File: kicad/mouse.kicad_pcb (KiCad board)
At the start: 2 copper layers, 100 x 100 mm, 49 parts, among them IC1 L7805, P1 SOURCE_12v, P10 LED_CONN, P11 SW_CONN, P12 LED_K_CONN, P15 UI_SOURCE, P16 LED_K_CONN, P17 LED_CONN, P18 SW_CONN, P2 SOURCE_12v, P3 battery 12v, P4 SOURCE_5v, P5 SOURCE_5v, P6 SOURCE_5v, P7 SOURCE_5v, P8 IR_CONN, P9 MOTOR_CONTROL, Q5 BSS138, Q6 BSS138, Q7 BSS138, SW1 SPST, SW2 SW_PUSH, SW3 SW_PUSH, SW4 SW_PUSH, SW5 SPST, U1 MCP3008

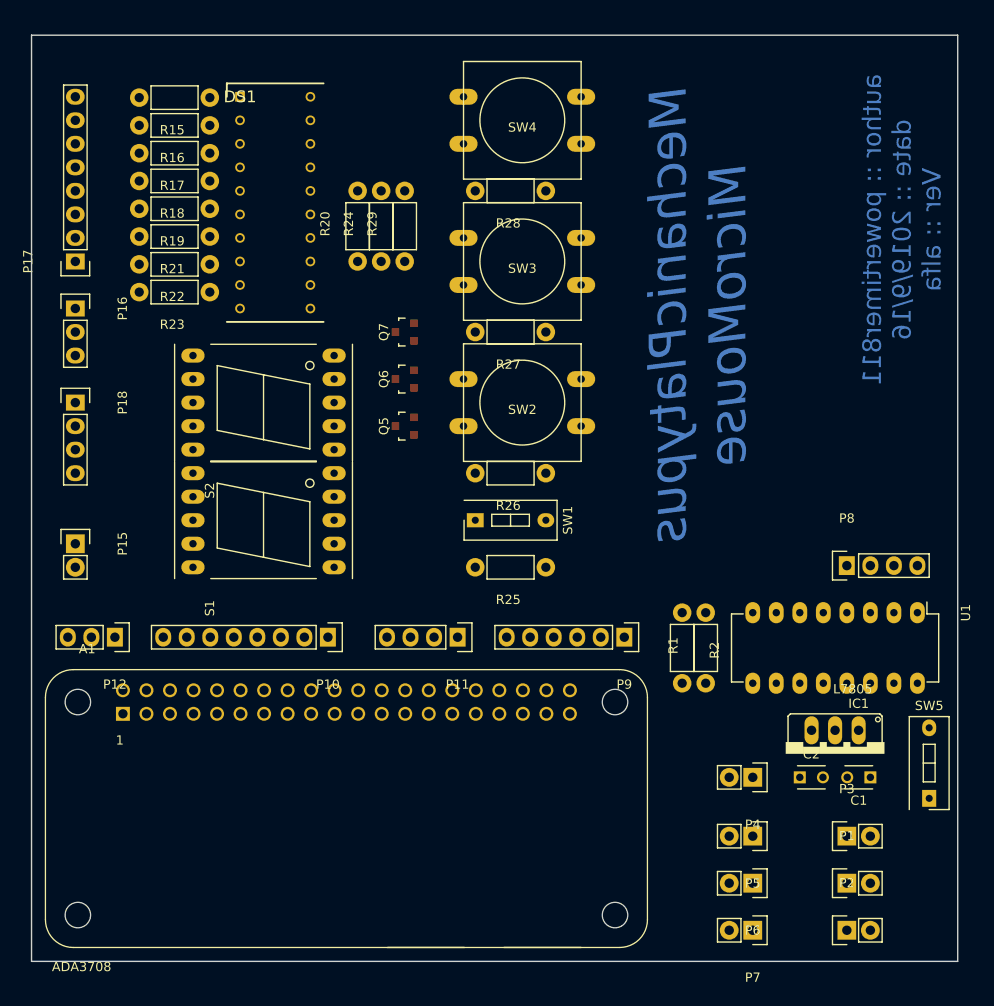
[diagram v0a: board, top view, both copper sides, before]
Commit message: complate kicad
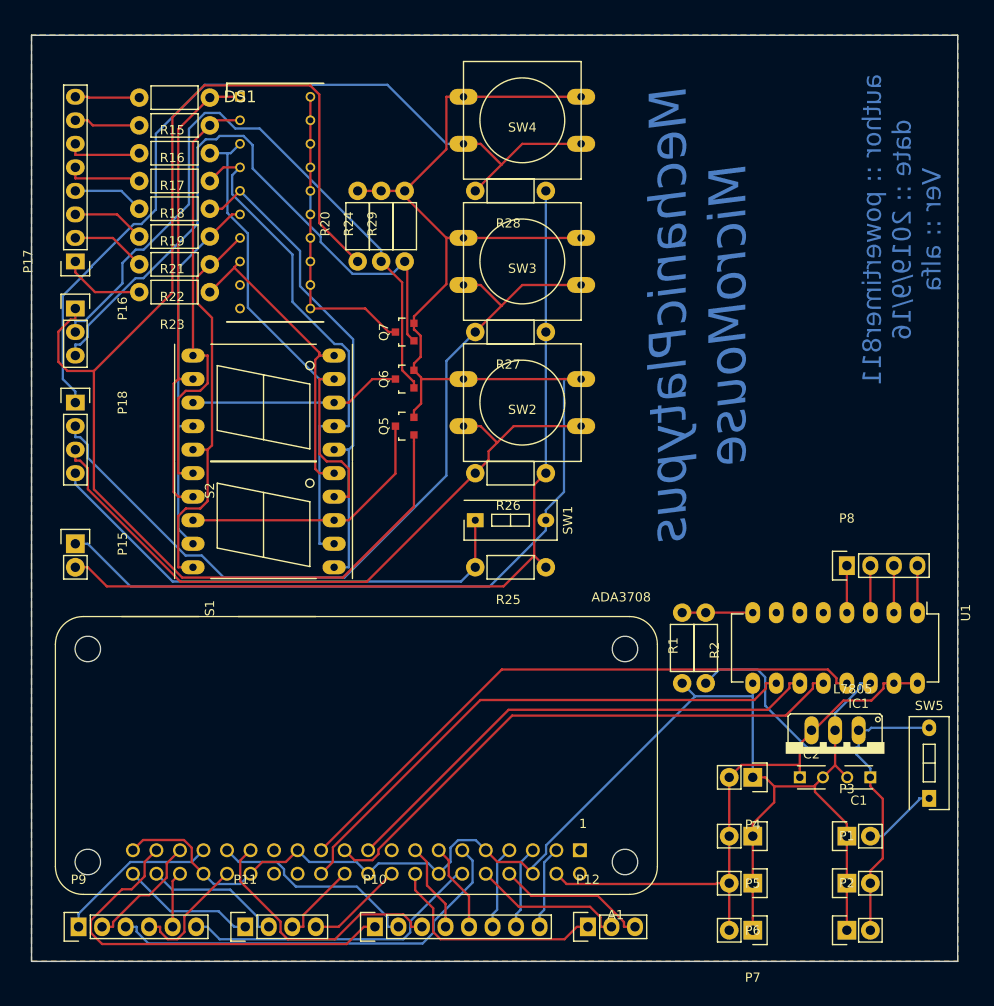
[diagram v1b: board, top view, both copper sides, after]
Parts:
- moved P9 66.7 mm to (30.1, 166.3), turned to 0 degrees
- moved P12 59.9 mm to (85.1, 166.3), turned to 0 degrees
- moved P11 38.8 mm to (48.1, 166.3), turned to 0 degrees
- moved P10 31.7 mm to (62.1, 166.3), turned to 0 degrees
- moved A1 17.3 mm to (60.1, 159.3), turned to 180 degrees
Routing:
- net Net-(P15-Pad1): track 0.00 -> 166.7 mm
- net GND: track 0.00 -> 155.4 mm
- net Net-(P16-Pad1): track 0.00 -> 141.6 mm
- net Net-(P15-Pad2): track 0.00 -> 93.4 mm
- net Net-(P18-Pad1): track 0.00 -> 90.8 mm
- net Net-(P18-Pad2): track 0.00 -> 88.3 mm
- net Net-(P18-Pad3): track 0.00 -> 74.4 mm
- net Net-(P16-Pad2): track 0.00 -> 72.1 mm
- net Net-(P16-Pad3): track 0.00 -> 69.1 mm
- net Net-(A1-Pad23): track 0.00 -> 65.8 mm
- net +5V: track 0.00 -> 63.4 mm
- net Net-(A1-Pad21): track 0.00 -> 60.7 mm
- net Net-(A1-Pad24): track 0.00 -> 58.9 mm
- net Net-(DS1-Pad4): track 0.00 -> 55.3 mm
- net Net-(P18-Pad4): track 0.00 -> 54.4 mm
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- added copper zone on B.Cu, net GND
- added copper zone on F.Cu, net GND
